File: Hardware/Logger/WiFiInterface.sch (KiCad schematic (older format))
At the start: 21 parts, among them J5 Conn_01x04_Female, Q1 FDV304P, Q2 FDV304P, U1 ESP-12E

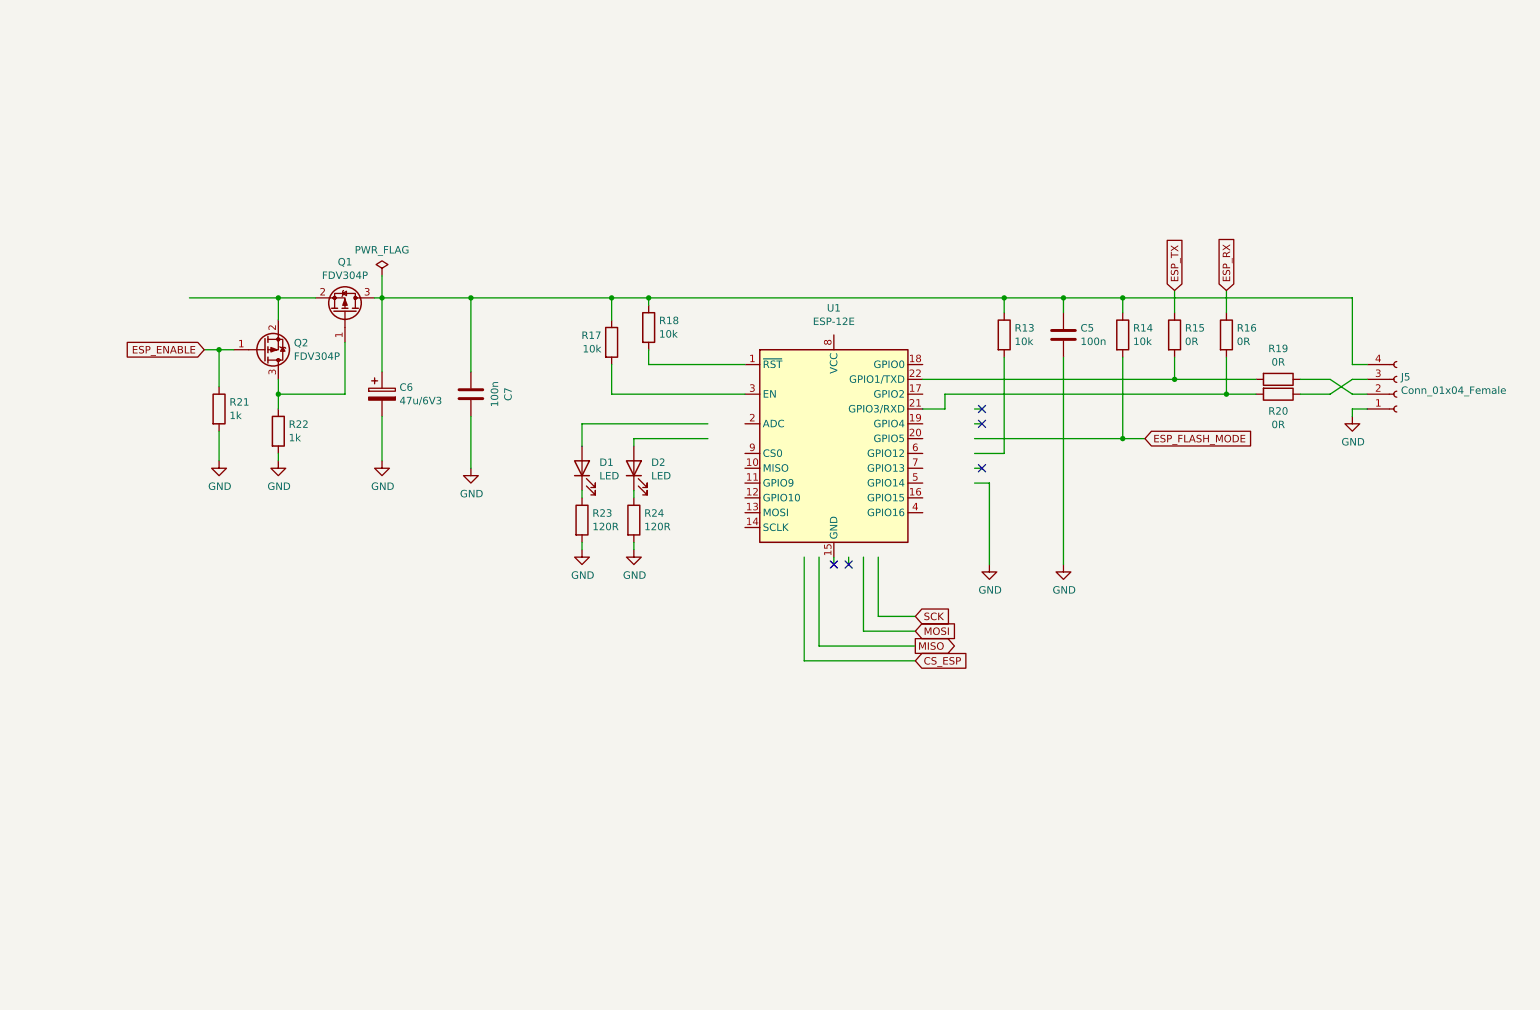
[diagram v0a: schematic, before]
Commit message: fix #27, fix #30, fix #32
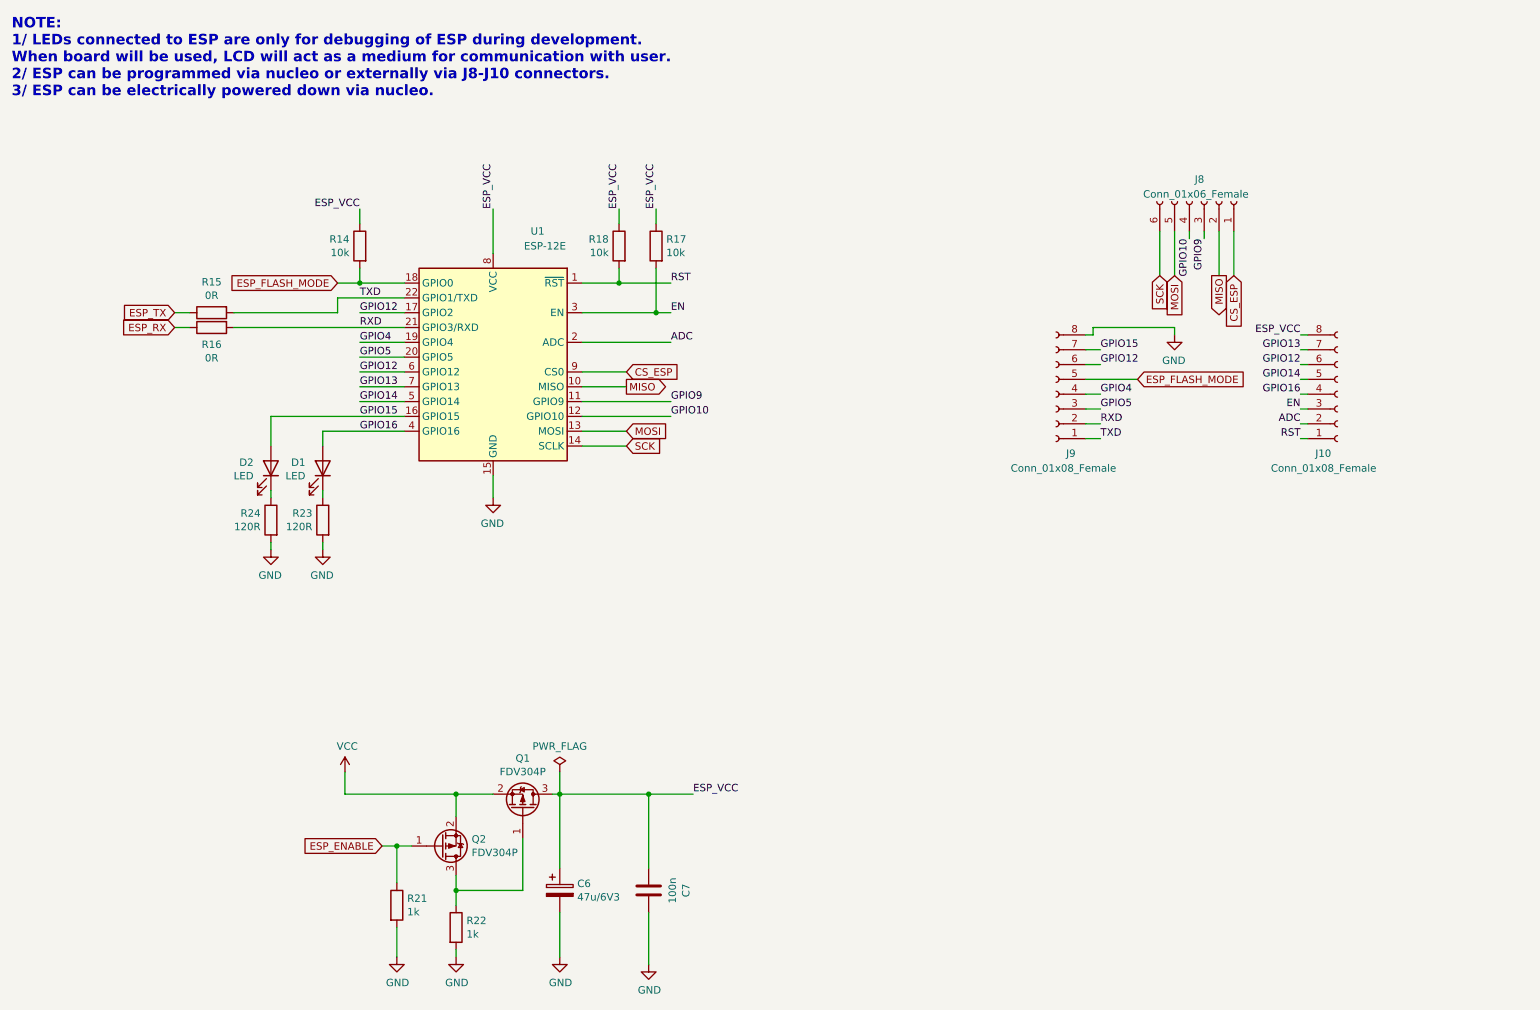
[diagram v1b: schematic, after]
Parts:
- removed C5: 100n, Capacitor_SMD:C_0402_1005Metric, symbol Device:C
- removed J5: Conn_01x04_Female, Connector_PinHeader_2.54mm:PinHeader_1x04_P2.54mm_Vertical, symbol Connector:Conn_01x04_Female
- removed R13: 10k, Resistor_SMD:R_0402_1005Metric, symbol Device:R
- removed R19, R20: 0R, Resistor_SMD:R_0402_1005Metric, symbol Device:R
- added J10, J9: Conn_01x08_Female, Connector_PinSocket_2.54mm:PinSocket_1x08_P2.54mm_Vertical, symbol Connector:Conn_01x08_Female
- added J8: Conn_01x06_Female, Connector_PinSocket_2.54mm:PinSocket_1x06_P2.54mm_Vertical, symbol Connector:Conn_01x06_Female
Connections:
- net labels added: ADC, EN, ESP_VCC, GPIO10, GPIO12, GPIO13, GPIO14, GPIO15, GPIO16, GPIO4, GPIO5, GPIO9, RST, RXD, TXD, VCC
- wire segments 83 -> 87
- no-connect marks 5 -> 0
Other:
- note added: "NOTE: \n1/ LEDs connected to ESP are only for debugging of ESP during development.\nWhen board will be used, LCD will act as a medium for communication with user.\n2/ ESP can be programmed via nucleo or externally via J8-J10 connectors.\n3/ ESP can be electrically powered down via nucleo."
- moved on the sheet: C6, C7, D1, D2, Q1, Q2, R14, R15, R16, R17, R18, R21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
